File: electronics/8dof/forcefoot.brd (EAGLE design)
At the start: 120 x 32 mm, 121 parts

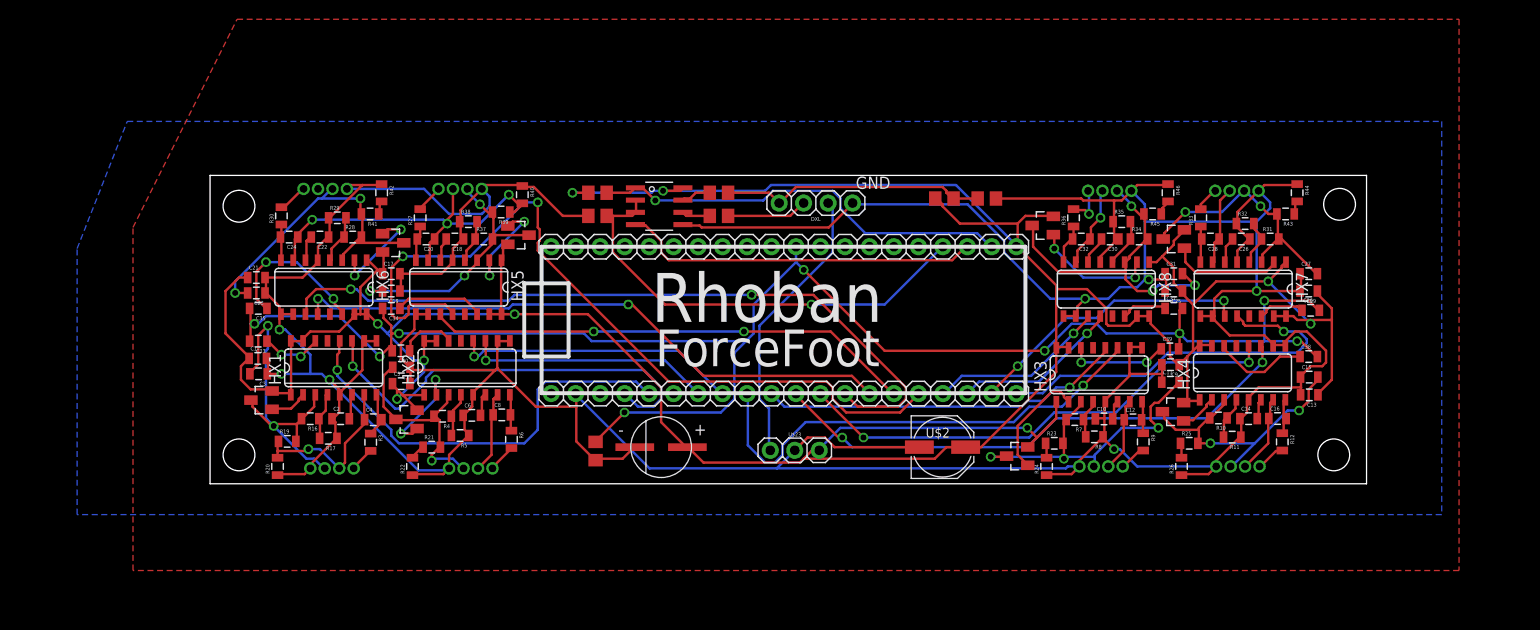
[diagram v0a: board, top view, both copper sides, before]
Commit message: Update schema
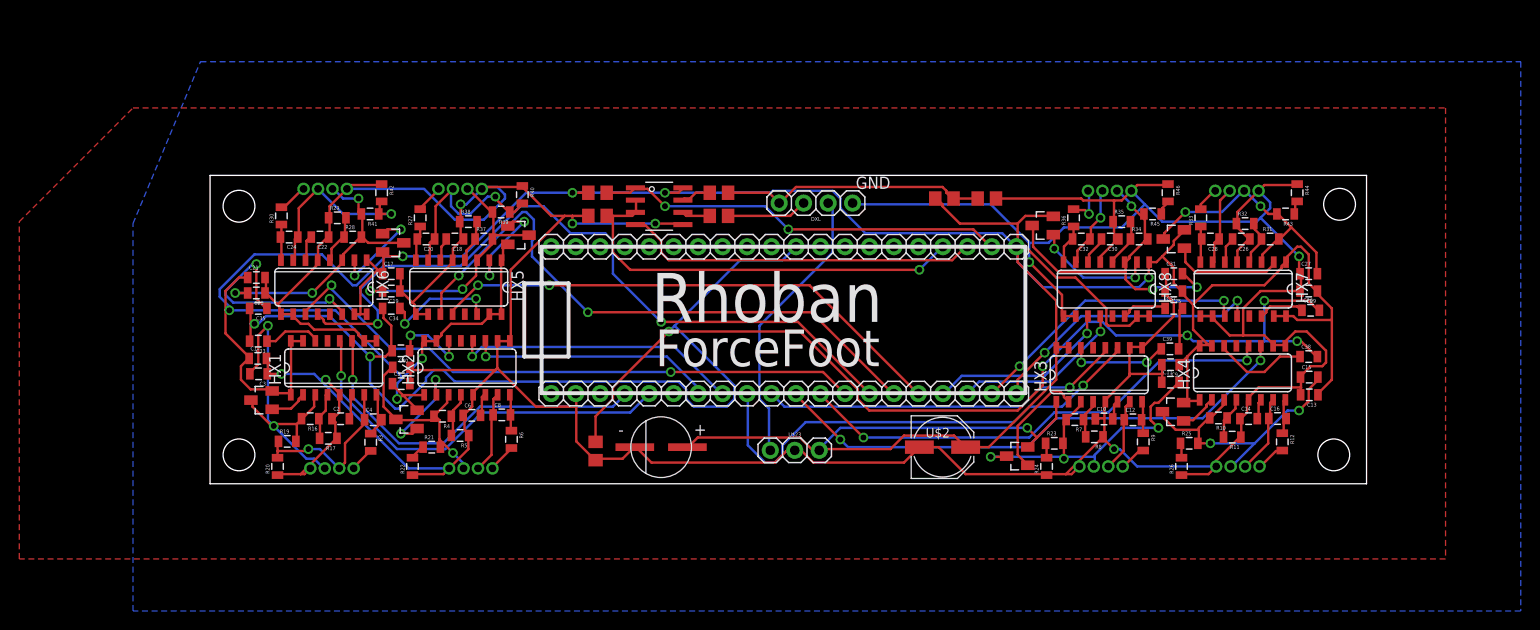
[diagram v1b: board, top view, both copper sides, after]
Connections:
- removed net 1A-4: R41.1, R42.2
- removed net N$15: U$18.P$3
- new net 5A-: C24.1, HX6.7, R41.1, R42.2, U$18.P$3
- net 6A-: no longer C24.1, HX6.7
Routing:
- net VCC: track 361.5 -> 401.5 mm, vias 9 -> 8
- net CLOCK: track 172.8 -> 206.5 mm, vias 9 -> 7
- net DOUT6: track 84.2 -> 54.5 mm
- net 5A-: track 0.00 -> 20.0 mm, vias 0 -> 1
- net 6A-: track 39.5 -> 20.3 mm, vias 3 -> 1
- net GND: track 495.2 -> 476.0 mm, vias 7 -> 8
- net SCK5: track 77.5 -> 62.3 mm
- net DOUT5: track 63.3 -> 77.5 mm
- net SCK6: track 50.7 -> 63.0 mm
- net DOUT8: track 41.0 -> 29.4 mm, vias 1 -> 2
- net N$18: track 16.3 -> 23.4 mm
- net SCK1: track 45.0 -> 38.3 mm
- net AVDD$5: track 33.3 -> 29.4 mm, vias 2 -> 3
- net DIRECTION: track 47.3 -> 44.3 mm
- net DOUT1: track 45.0 -> 42.3 mm
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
